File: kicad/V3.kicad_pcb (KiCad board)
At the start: 2 copper layers, 180.5 x 123.2 mm, 61 parts, among them SW1 KS33_SW_HS, SW10 KS33_SW_HS, SW11 KS33_SW_HS, SW12 KS33_SW_HS, SW13 KS33_SW_HS, SW14 KS33_SW_HS, SW15 KS33_SW_HS, SW16 KS33_SW_HS, SW17 KS33_SW_HS, SW18 KS33_SW_HS, SW19 KS33_SW_HS, SW2 KS33_SW_HS, SW20 KS33_SW_HS, SW21 KS33_SW_HS, SW22 KS33_SW_HS, SW23 KS33_SW_HS, SW3 KS33_SW_HS, SW4 KS33_SW_HS, SW5 KS33_SW_HS, SW6 KS33_SW_HS, SW7 KS33_SW_HS, SW8 KS33_SW_HS, SW9 KS33_SW_HS, U2 CH9329, U3 USB_C_C393939, U4 SSD1306-128X64-OLED-0.96

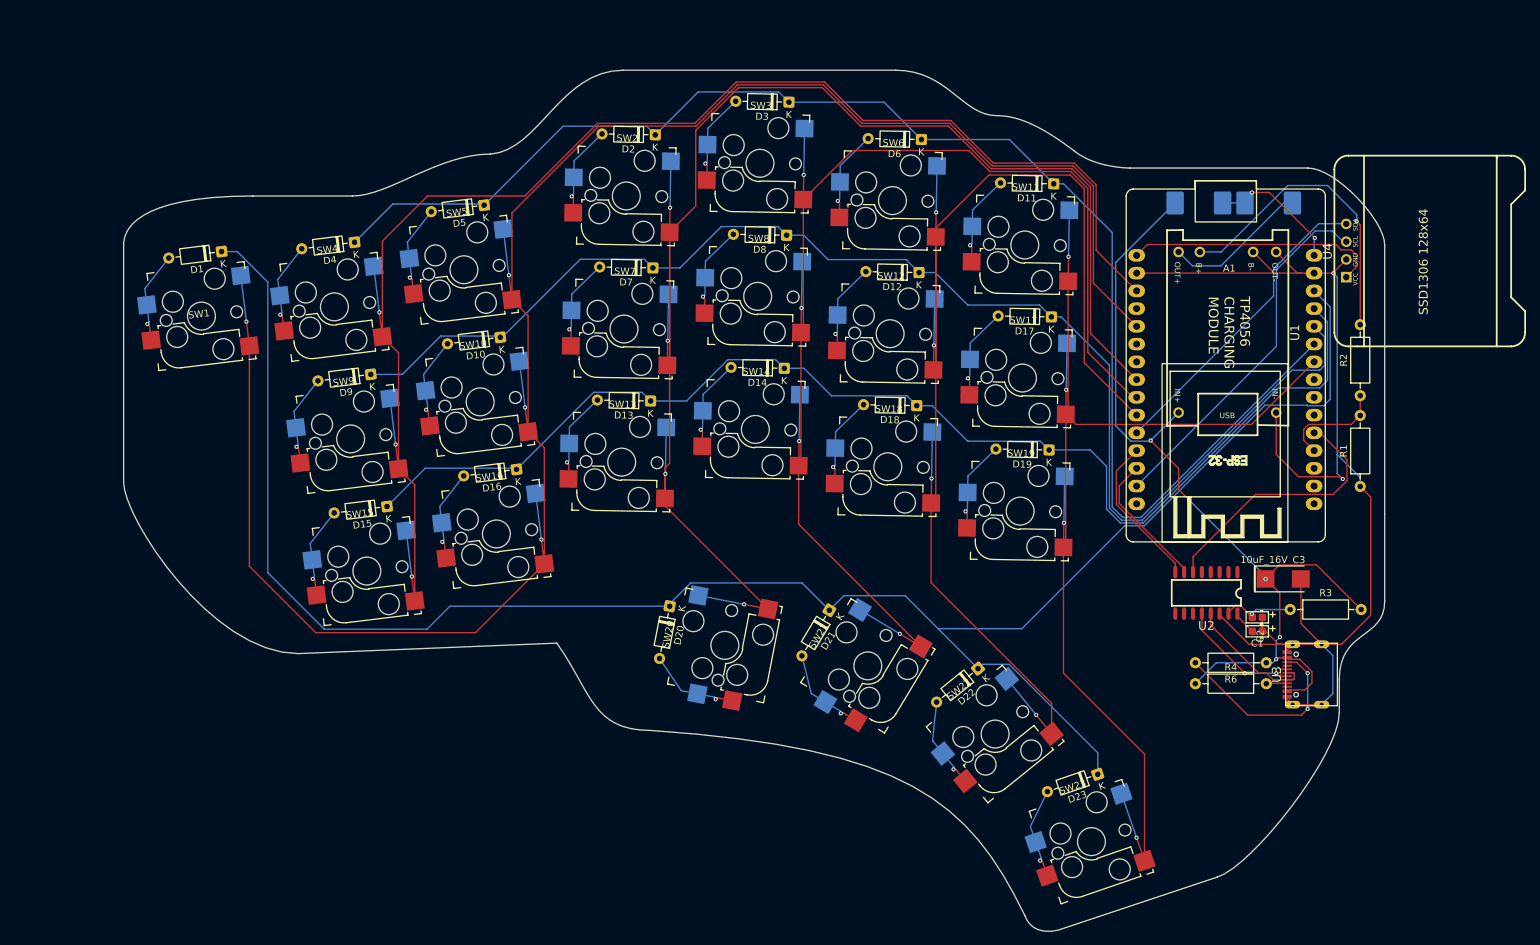
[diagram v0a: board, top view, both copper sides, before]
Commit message: working version
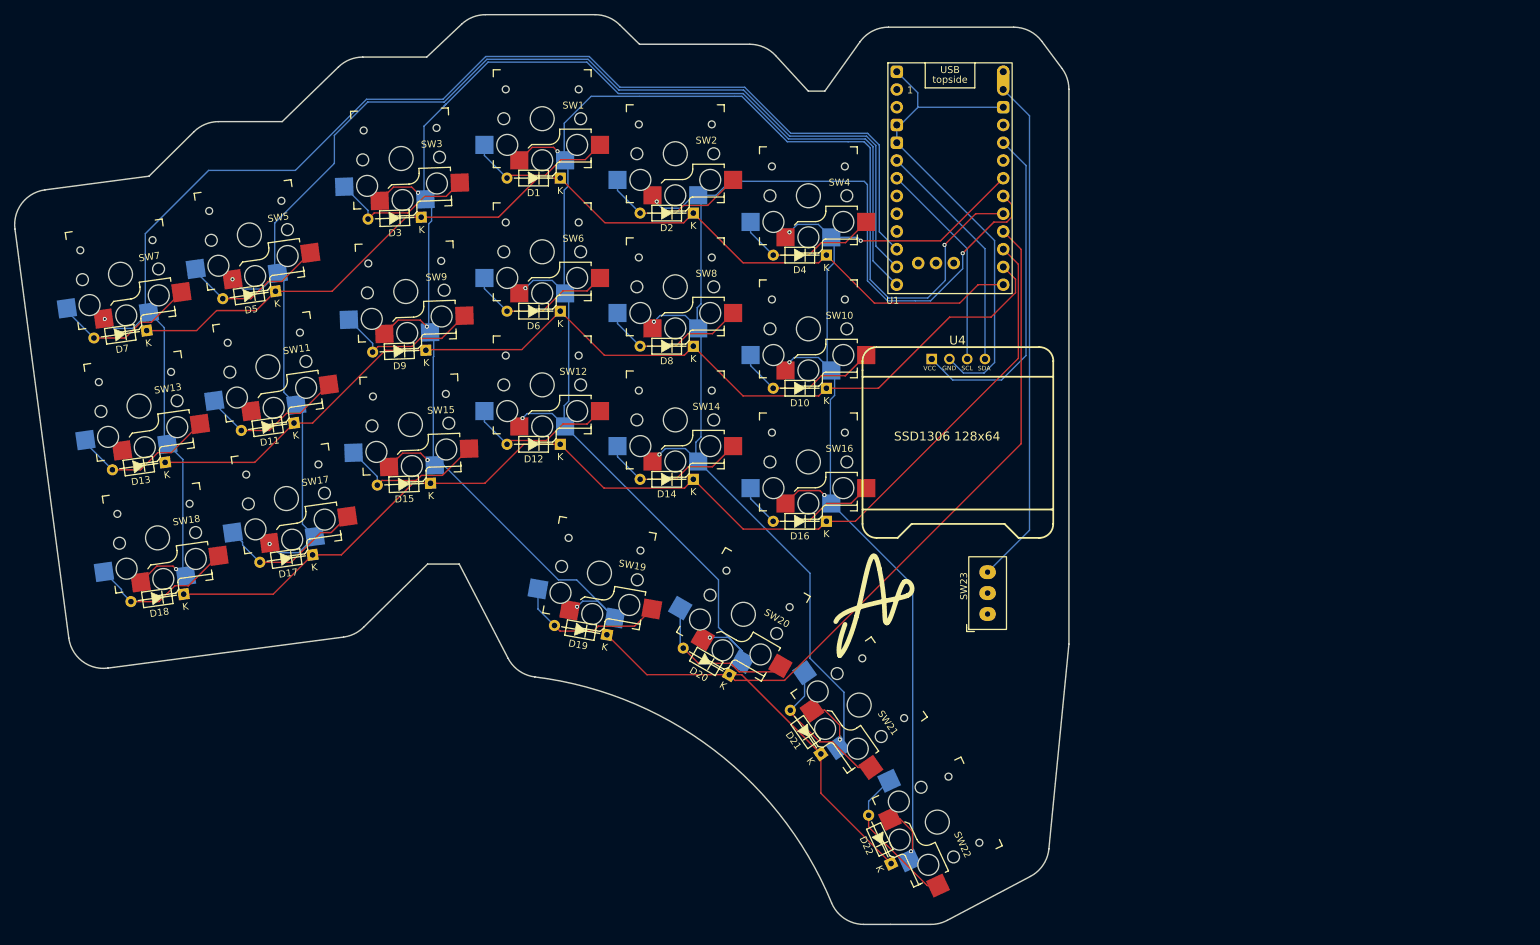
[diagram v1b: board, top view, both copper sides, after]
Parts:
- removed A1: ESP32_DevKit_V1_DOIT_30GPIOs, PCM_SL_Development_Boards:DOIT_ESP32_DEVKIT_30Pins
- removed C1, C2: 0.1uF_0603_16V, PCM_Capacitor_Tantalum_SMD_Handsoldering_AKL:CP_EIA-1608-08_AVX-J
- removed C3: 10uF_16V, PCM_4ms_Capacitor:CP_Tantalum_EIA-6032-28_Kemet-C
- removed D23: 1N4148, Diode_THT:D_DO-35_SOD27_P7.62mm_Horizontal
- removed DS1, DS2: SS34, PCM_Diode_SMD_AKL:D_SMC
- removed R1: 270k, Resistor_THT:R_Axial_DIN0207_L6.3mm_D2.5mm_P10.16mm_Horizontal
- removed R2: 100k, Resistor_THT:R_Axial_DIN0207_L6.3mm_D2.5mm_P10.16mm_Horizontal
- removed R3: 1R, Resistor_THT:R_Axial_DIN0207_L6.3mm_D2.5mm_P10.16mm_Horizontal
- removed R4, R6: 5.1k, Resistor_THT:R_Axial_DIN0207_L6.3mm_D2.5mm_P10.16mm_Horizontal
- removed U2: CH9329, Library:CH9329
- removed U3: USB_C_C393939, Library:USBC_C393939
- D1, D10, D11, D12, D13, D14, D15, D16, D17, D18, D19, D2, D20, D21, D22, D3, D4, D5, D6, D7, D8, D9: footprint Diode_THT:D_DO-35_SOD27_P7.62mm_Horizontal -> PCM_Diode_THT_AKL:D_DO-35_SOD27_P7.62mm_Horizontal
- SW1, SW10, SW11, SW12, SW13, SW14, SW15, SW16, SW17, SW18, SW19, SW2, SW20, SW21, SW22, SW3, SW4, SW5, SW6, SW7, SW8, SW9: footprint keyswitches:Kailh_socket_MX_reversible -> keyswitches:Kailh_socket_PG1350_reversible
- SW23: value KS33_SW_HS -> Slide_Switch_SPDT_P3mm_10x5x10mm; footprint keyswitches:Kailh_socket_MX_reversible -> PCM_SL_Devices:Slide_Switch_SPDT_P3mm_10x5x10mm
- U1: value ~ -> SuperMini nRF52840; footprint Library:HAYATEC TP4056 LIPO CHARGING MODULE -> PCM_marbastlib-xp-promicroish:SuperMini_nRF52840_AH_USBup
- moved D11 114.0 mm to (76.9, 88.5), turned to -172 degrees
- moved D17 111.1 mm to (79.5, 107.4), turned to -172 degrees
- moved SW11 109.7 mm to (73.2, 80.4), turned to 8 degrees
- moved D18 108.3 mm to (61.1, 113.0), turned to -172 degrees
- moved SW17 106.8 mm to (75.8, 99.3), turned to 8 degrees
- moved SW18 105.0 mm to (57.4, 104.9), turned to 8 degrees
- moved U4 98.7 mm to (158.3, 104.9), turned to 0 degrees
- moved D7 73.0 mm to (55.8, 75.3), turned to -172 degrees
- moved SW7 72.5 mm to (52.1, 67.2), turned to 8 degrees
- moved D13 70.0 mm to (58.4, 94.1), turned to -172 degrees
- moved SW4 69.7 mm to (150.5, 56.0), turned to 0 degrees
- moved SW13 69.5 mm to (54.7, 86.1), turned to 8 degrees
- moved D19 68.6 mm to (121.7, 118.8), turned to 170 degrees
- moved D4 67.6 mm to (153.1, 64.5), turned to 180 degrees
- moved SW19 60.9 mm to (120.6, 110.0), turned to -10 degrees
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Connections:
- D1 pad 1: /Row4 -> /Row1
- D11 pad 1: /Row1 -> /Row2
- D12 pad 1: /Row2 -> /Row3
- D13 pad 1: /Row3 -> /Row2
- D17 pad 1: /Row2 -> /Row3
- D19 pad 1: /Row3 -> /Row4
- D6 pad 1: /Row1 -> /Row2
- D7 pad 1: /Row2 -> /Row1
- SW1 pad 1: /Col2 -> /Col4
- SW10 pad 1: /Col2 -> /Col6
- SW11 pad 1: /Col6 -> /Col2
- SW12 pad 1: /Col5 -> /Col4
- SW13 pad 1: /Col3 -> /Col1
- SW14 pad 1: /Col4 -> /Col5
- SW15 pad 1: /Col1 -> /Col3
- SW16 pad 1: /Col2 -> /Col6
- SW17 pad 1: /Col6 -> /Col2
- SW18 pad 1: /Col5 -> /Col1
- SW19 pad 1: /Col6 -> /Col3
- SW2 pad 1: /Col3 -> /Col5
- SW20 pad 1: /Col3 -> /Col4
- SW21 pad 1: /Col4 -> /Col5
- SW22 pad 1: /Col5 -> /Col6
- SW23 pad 1: /Col6 -> Net-(BT1-+)
- SW23 pad 2: Net-(D23-A) -> unconnected-(SW23-Pad2)
- SW3 pad 1: /Col4 -> /Col3
- SW4 pad 1: /Col1 -> /Col6
- SW6 pad 1: /Col5 -> /Col4
- SW7 pad 1: /Col3 -> /Col1
- SW8 pad 1: /Col4 -> /Col5
- SW9 pad 1: /Col1 -> /Col3
- U1 pad 1: Earth -> unconnected-(U1-P0.06-Pad1)
- U1 pad 2: +5V -> unconnected-(U1-P0.08-Pad2)
- U1 pad 5: /B+ -> /SDA
- U1 pad 6: Net-(DS2-A) -> /SCL
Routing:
- net /Row4: track 276.7 -> 145.1 mm
- net +5V: track 128.5 -> 0.00 mm, vias 5 -> 0
- net /Col2: track 294.0 -> 185.1 mm, vias 4 -> 2
- net Earth: track 171.7 -> 70.4 mm, vias 2 -> 0
- net /Row1: track 205.9 -> 142.2 mm
- net /Row2: track 191.2 -> 147.3 mm
- net /USB_rst: track 38.0 -> 0.00 mm
- net /B+: track 44.0 -> 73.1 mm, vias 1 -> 0
- net /HID connector/CC2: track 28.2 -> 0.00 mm, vias 2 -> 0
- net /Col3: track 231.5 -> 206.5 mm
- net /RX: track 22.1 -> 0.00 mm
- net /SCL: track 51.7 -> 30.1 mm
- net Net-(DS2-A): track 20.9 -> 0.00 mm
- net /TX: track 19.7 -> 0.00 mm
- net /Col4: track 191.1 -> 210.2 mm, vias 4 -> 5
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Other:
- board size 180.5 x 123.2 mm -> 150.9 x 130.2 mm
